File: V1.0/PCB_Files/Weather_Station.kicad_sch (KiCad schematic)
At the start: 17 parts, among them SW1 SW_Push, U1 STM32F103C8T6, Y1 Crystal_GND24

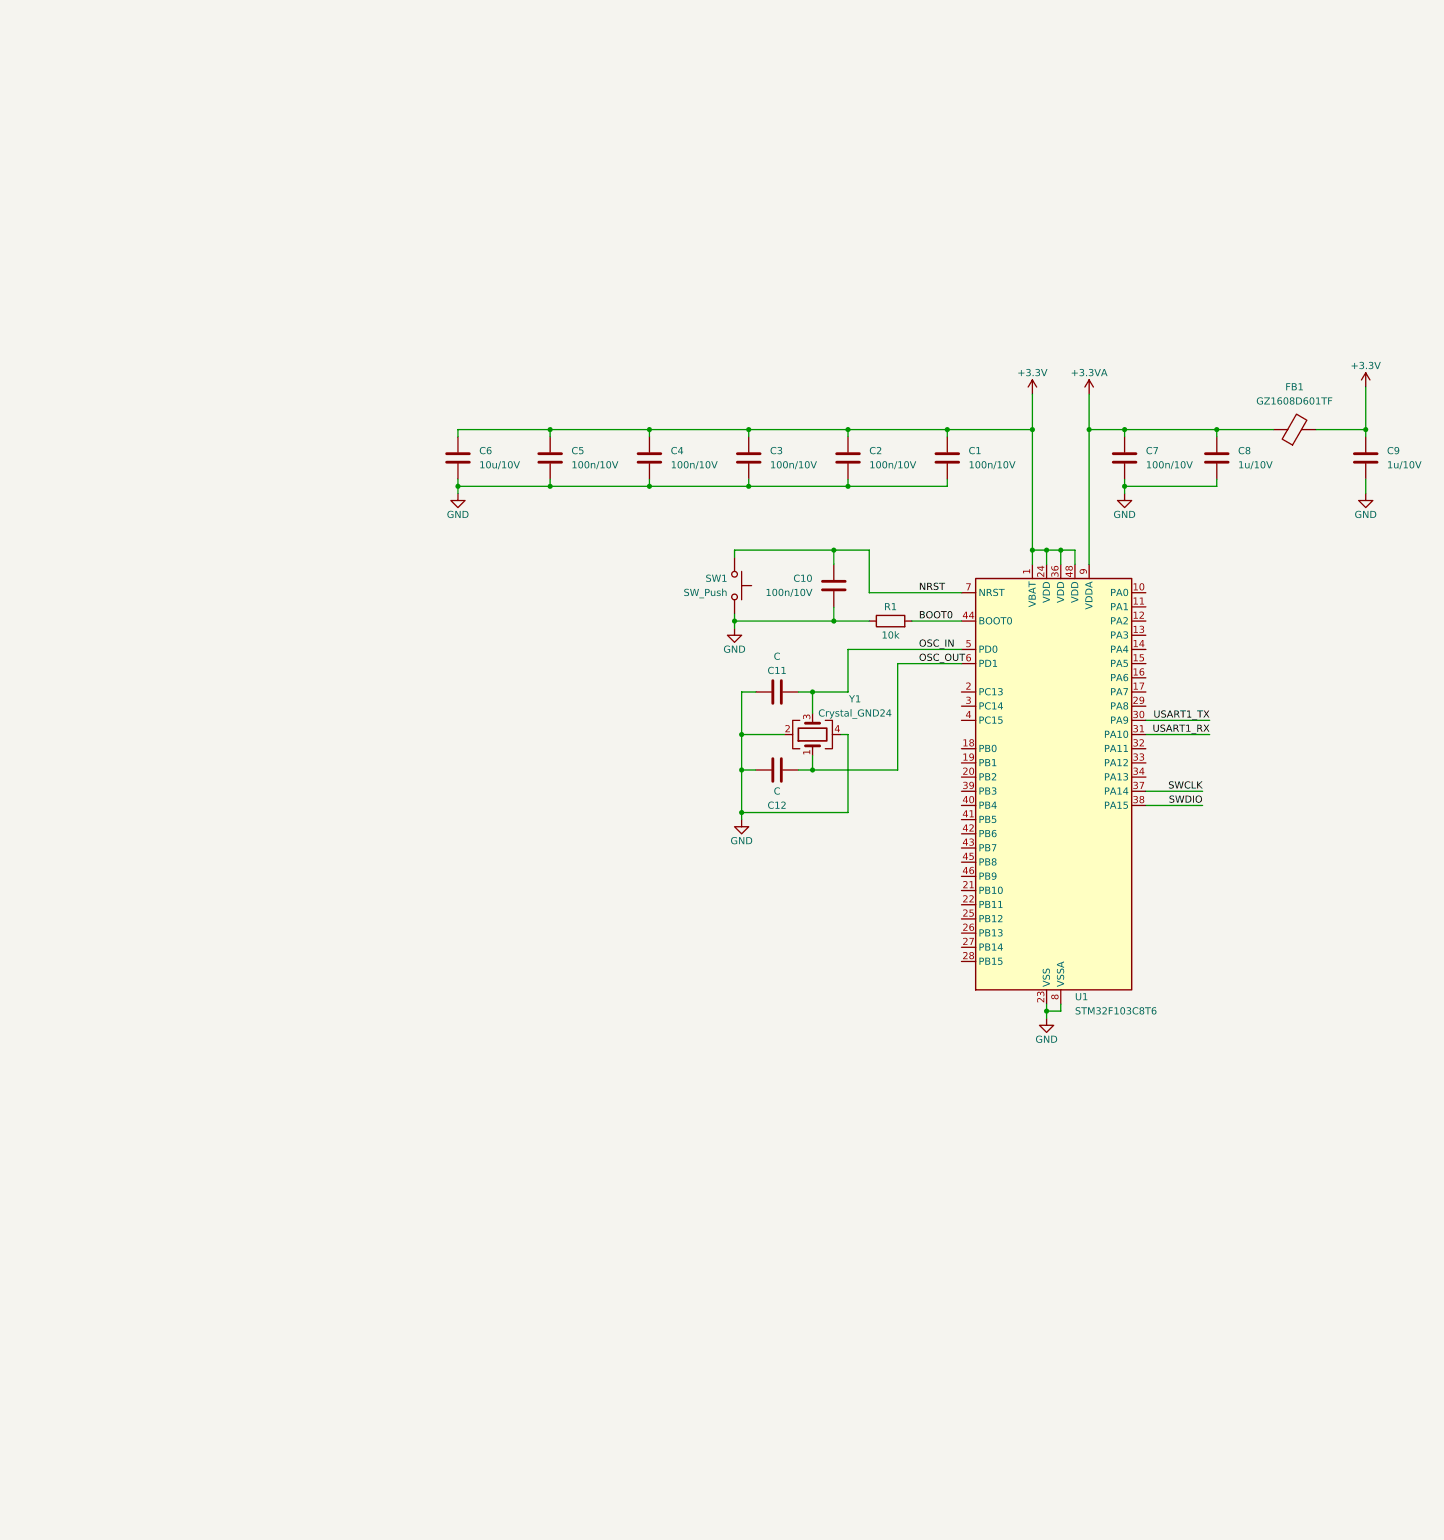
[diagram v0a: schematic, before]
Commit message: Some changes in the IOC and continues Schematic.
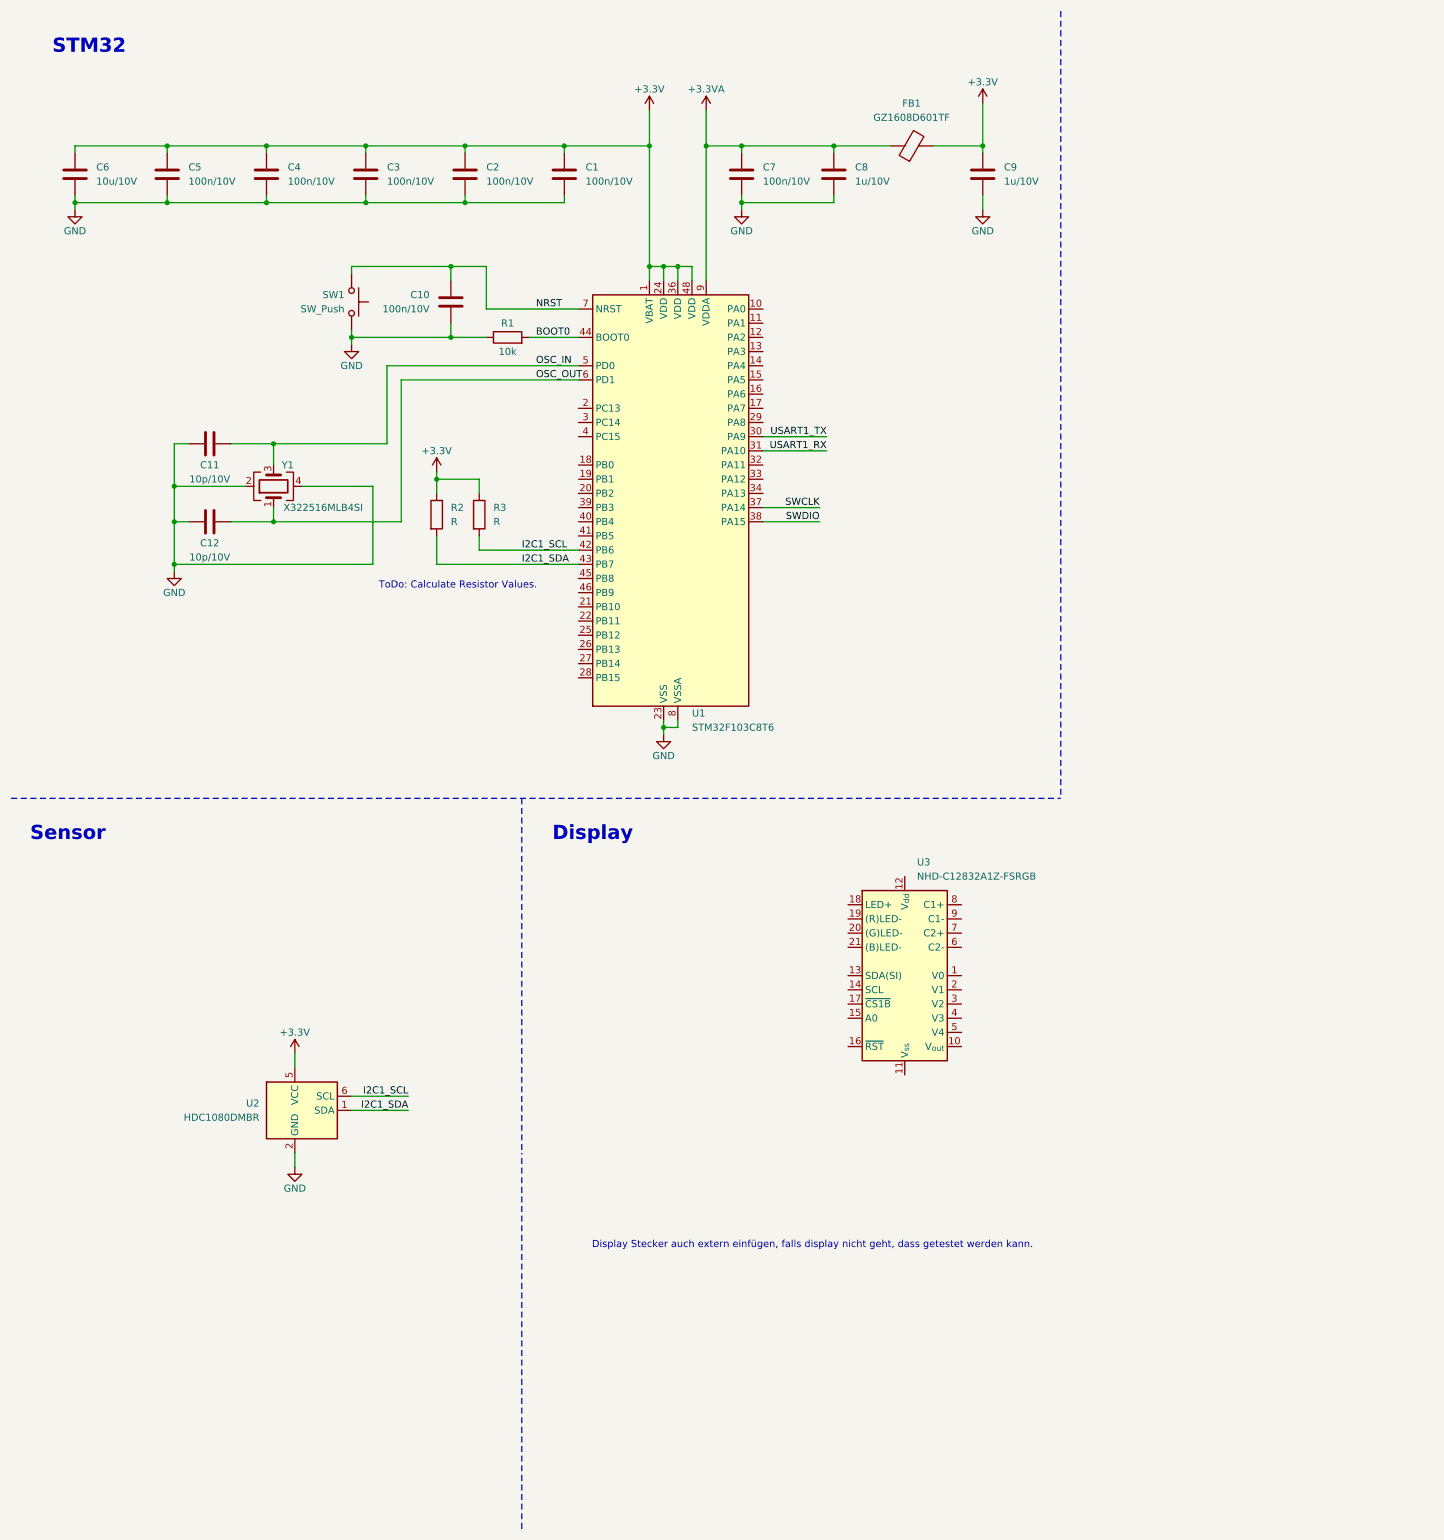
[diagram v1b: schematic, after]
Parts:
- added R2, R3: R, symbol Device:R
- added U2: HDC1080DMBR, Package_SON:Texas_PWSON-N6, symbol Sensor_Humidity:HDC1080
- added U3: NHD-C12832A1Z-FSRGB, Display:HY1602E, symbol Display_Graphic:NHD-C12832A1Z-FSRGB
- C11, C12: value C -> 10p/10V
- Y1: value Crystal_GND24 -> X322516MLB4SI
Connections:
- net +3.3V: now also R2.1, R3.1, U2.5 (VCC)
- net GND: now also C12.1, U2.2 (GND); no longer C12.2
- net OSC_OUT: now also C12.2; no longer C12.1
- net I2C1_SCL: now reaches U1.42 (PB6)
- net I2C1_SCL: now also R3.2, U2.6 (SCL)
- net I2C1_SDA: now reaches U1.43 (PB7)
- net I2C1_SDA: now also R2.2, U2.1 (SDA)
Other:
- note added: "Display"
- note added: "Display Stecker auch extern einfügen, falls display nicht geht, dass getestet werden kann."
- note added: "STM32"
- note added: "Sensor"
- note added: "ToDo: Calculate Resistor Values."
- moved on the sheet: C1, C10, C11, C2, C3, C4, C5, C6, C7, C8, C9, FB1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
